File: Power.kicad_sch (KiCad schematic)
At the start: 21 parts, among them J2 USB_C_Receptacle_USB2.0_16P, J3 Conn_01x02, Q1 AO3401A, U3 CN3063, U4 TLV74033PDBVR, U5 CH340N, U6 TPS7A0522PDBV

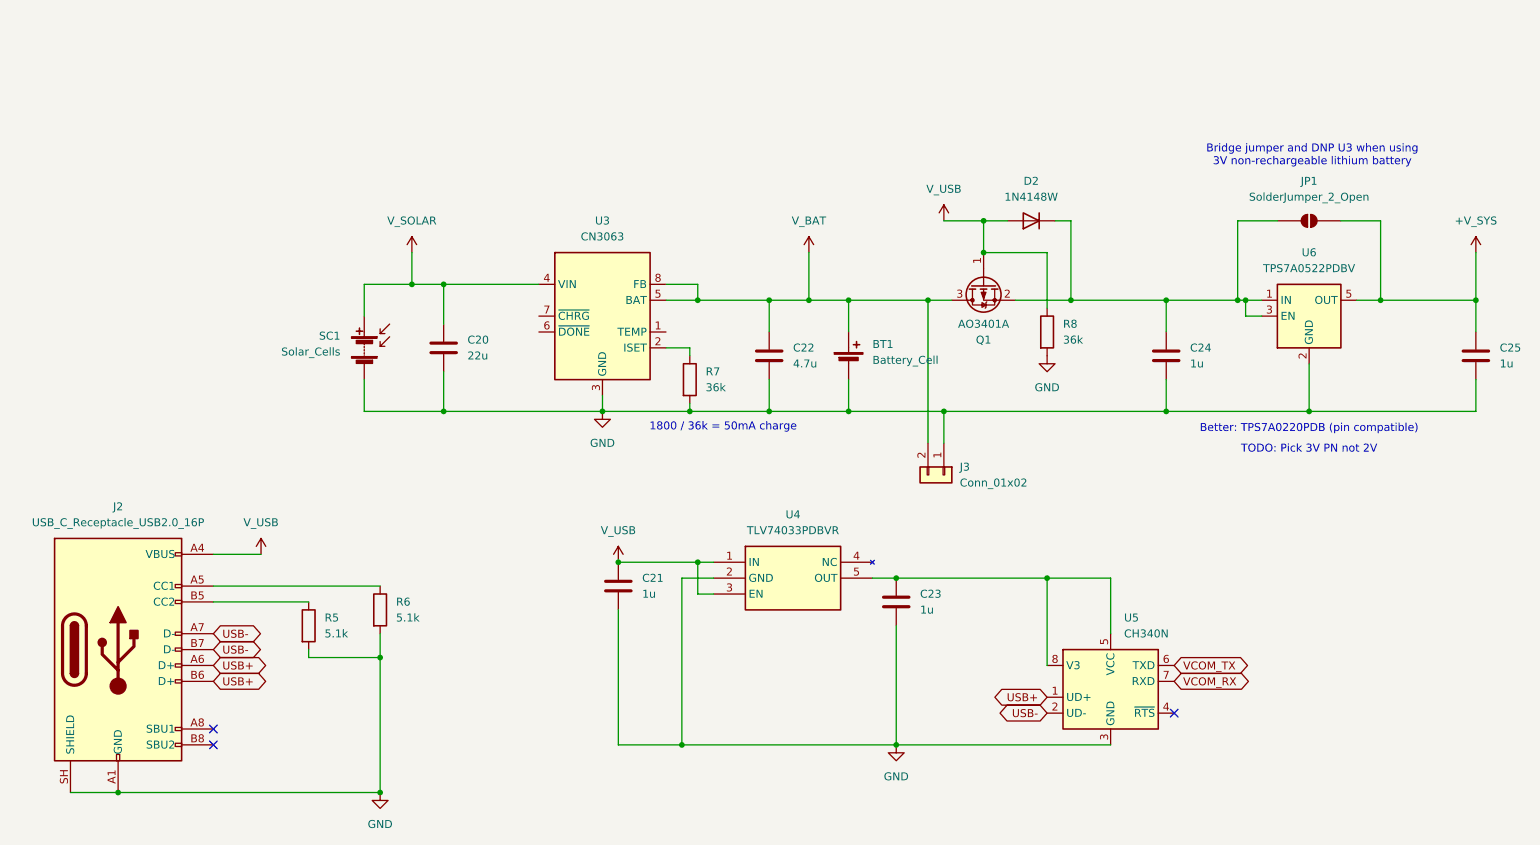
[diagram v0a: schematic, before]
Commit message: preliminary JLCPCB BOM, some initial changes for r1
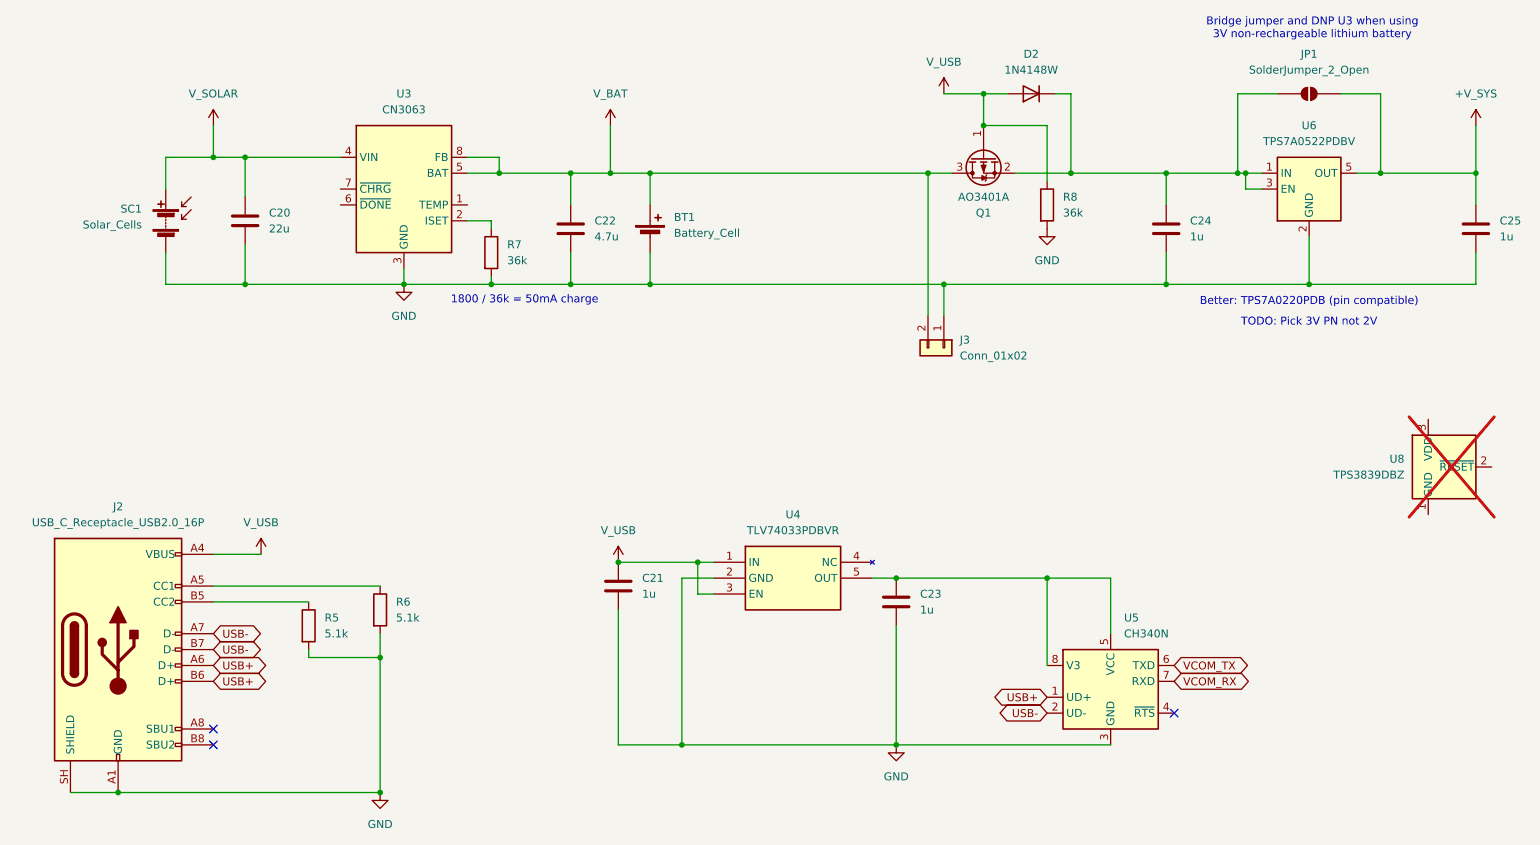
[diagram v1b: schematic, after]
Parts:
- added U8: TPS3839DBZ, Package_TO_SOT_SMD:SOT-23, symbol Power_Supervisor:TPS3839DBZ
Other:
- moved on the sheet: BT1, C20, C22, C24, C25, D2, J3, JP1, Q1, R7, R8, SC1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
